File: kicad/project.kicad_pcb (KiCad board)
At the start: 2 copper layers, 58.4 x 58.4 mm, 22 parts, among them J1 Conn_01x08_Pin, J2 PiZeroW_Bottom_Mount

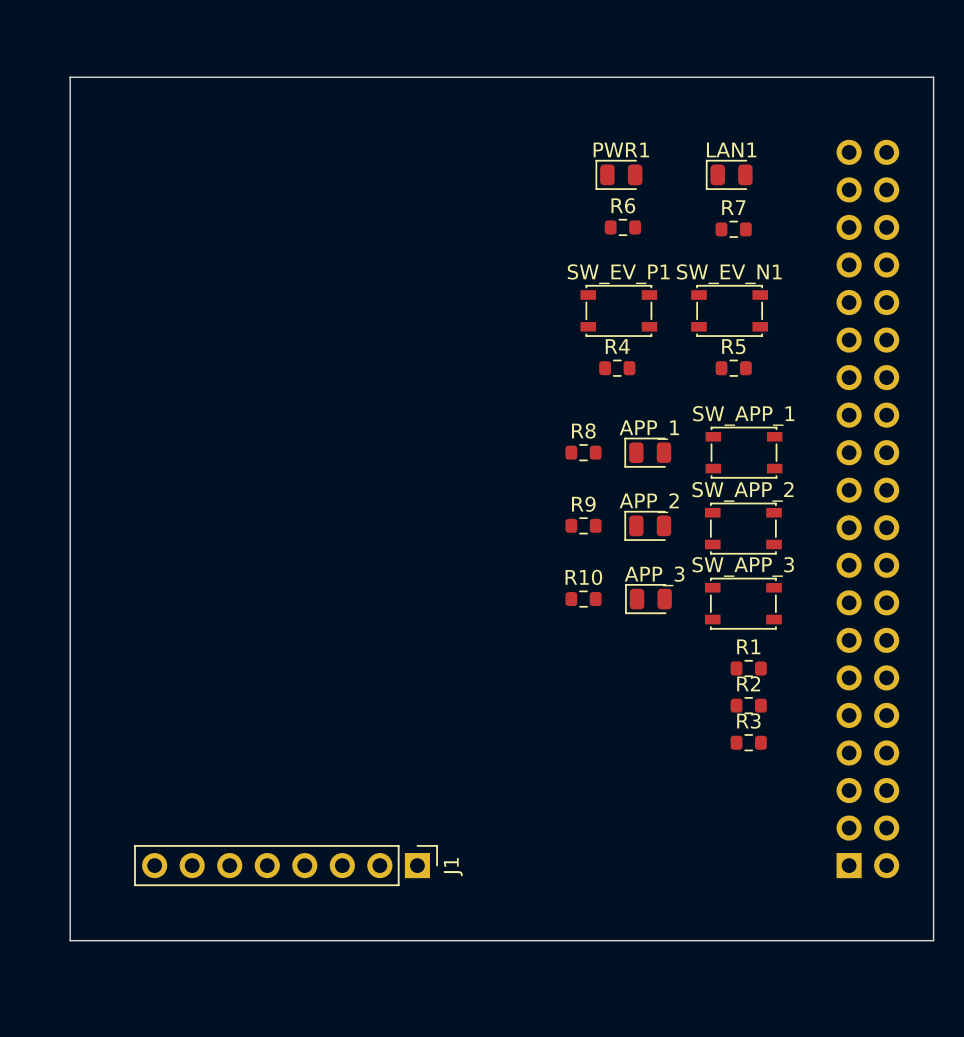
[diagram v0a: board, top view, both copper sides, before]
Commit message: completed board layout and passed drc
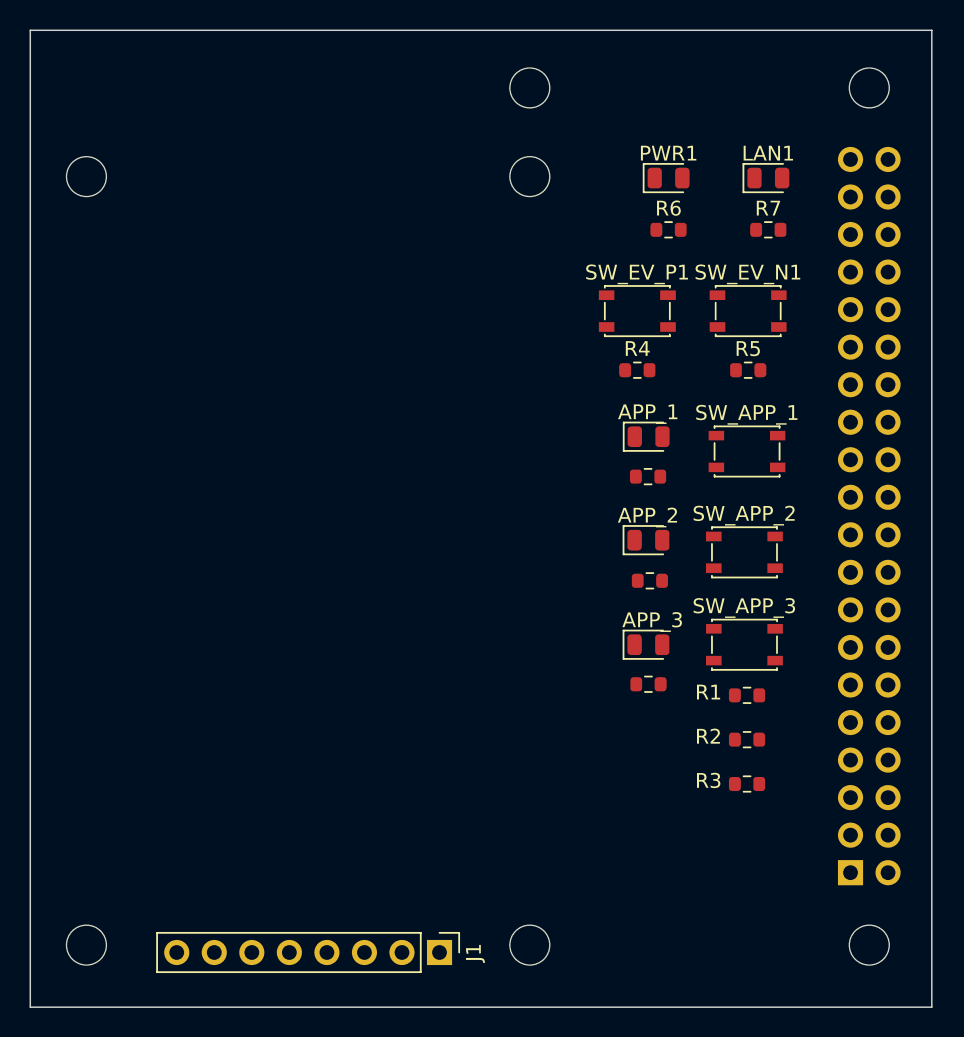
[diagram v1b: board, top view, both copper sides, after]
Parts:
- added REF**: MountingHole_2.7mm_M2.5, MountingHole:MountingHole_2.7mm_M2.5, F.Cu at (130.3, 43.9)
- added REF**: MountingHole_2.7mm_M2.5, MountingHole:MountingHole_2.7mm_M2.5, F.Cu at (77.3, 49.9)
- added REF**: MountingHole_2.7mm_M2.5, MountingHole:MountingHole_2.7mm_M2.5, F.Cu at (107.3, 49.9)
- added REF**: MountingHole_2.7mm_M2.5, MountingHole:MountingHole_2.7mm_M2.5, F.Cu at (107.3, 101.9)
- added REF**: MountingHole_2.7mm_M2.5, MountingHole:MountingHole_2.7mm_M2.5, F.Cu at (130.3, 101.9)
- added REF**: MountingHole_2.7mm_M2.5, MountingHole:MountingHole_2.7mm_M2.5, F.Cu at (107.3, 43.9)
- added REF**: MountingHole_2.7mm_M2.5, MountingHole:MountingHole_2.7mm_M2.5, F.Cu at (77.3, 101.9)
- moved R10 7.25 mm to (115.3, 84.2)
- moved J1 6.07 mm to (101.2, 102.4)
- moved R9 5.83 mm to (115.4, 77.2)
- moved R8 4.66 mm to (115.3, 70.2)
- moved PWR1 3.21 mm to (116.7, 50.0)
- moved APP_3 3.09 mm to (115.3, 81.6)
- moved R6 3.09 mm to (116.7, 53.5)
- moved R3 2.80 mm to (122.0, 91.0)
- moved SW_APP_3 2.78 mm to (121.8, 81.6)
- moved LAN1 2.49 mm to (123.4, 50.0)
- moved R7 2.34 mm to (123.4, 53.5)
- moved R2 2.31 mm to (122.0, 88.0)
- moved R1 1.82 mm to (122.0, 85.0)
- moved SW_APP_2 1.61 mm to (121.8, 75.3)
- moved R4 1.36 mm to (114.6, 63.0)
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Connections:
- J1 pad 3: unconnected-(J1-Pin_3-Pad3) -> /LCD_Display/LCD_SCL
- J1 pad 4: unconnected-(J1-Pin_4-Pad4) -> /LCD_Display/LCD_SDA
- J1 pad 5: unconnected-(J1-Pin_5-Pad5) -> /LCD_Display/LCD_RES
- J1 pad 6: unconnected-(J1-Pin_6-Pad6) -> /LCD_Display/LCD_DC
- J1 pad 7: unconnected-(J1-Pin_7-Pad7) -> /LCD_Display/LCD_CS
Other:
- board size 58.4 x 58.4 mm -> 61 x 66.1 mm
